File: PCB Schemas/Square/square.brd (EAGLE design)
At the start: 100 x 80 mm, 10 parts

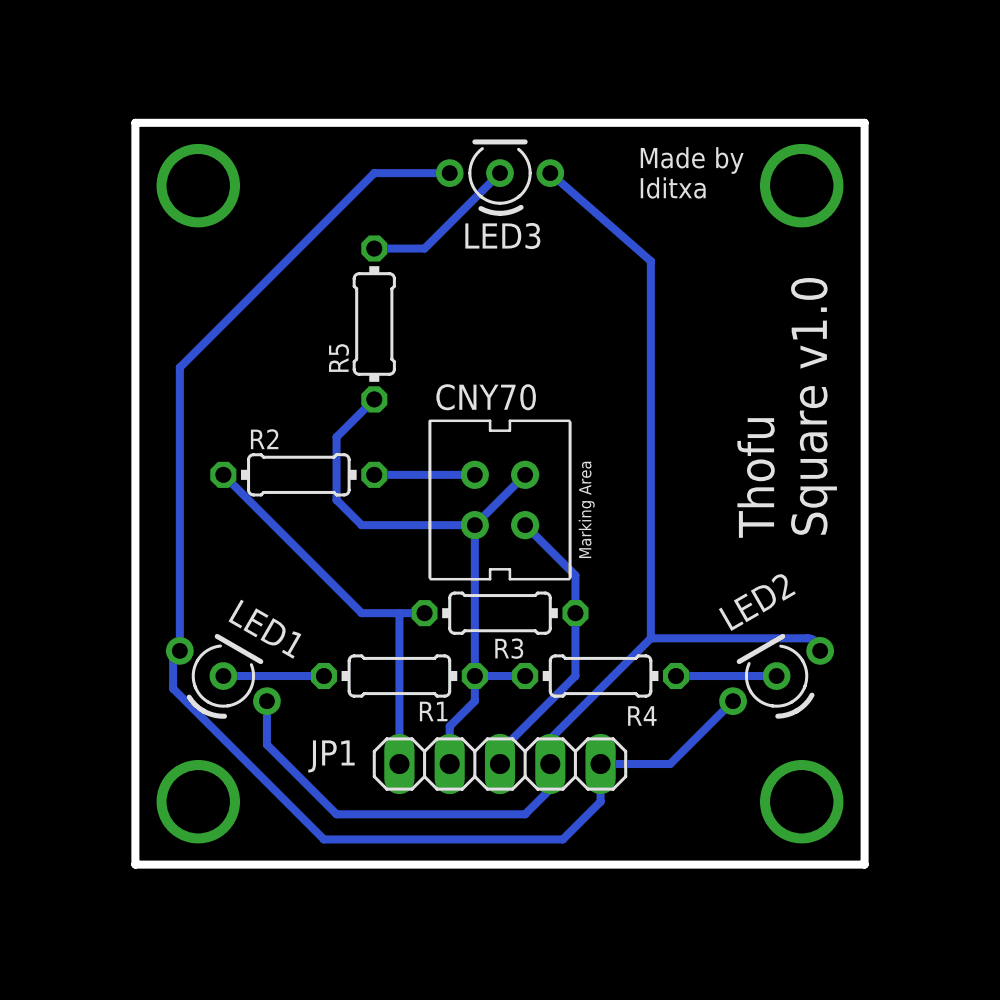
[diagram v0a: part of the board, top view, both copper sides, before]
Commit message: Updated and Finalized Square Board V1
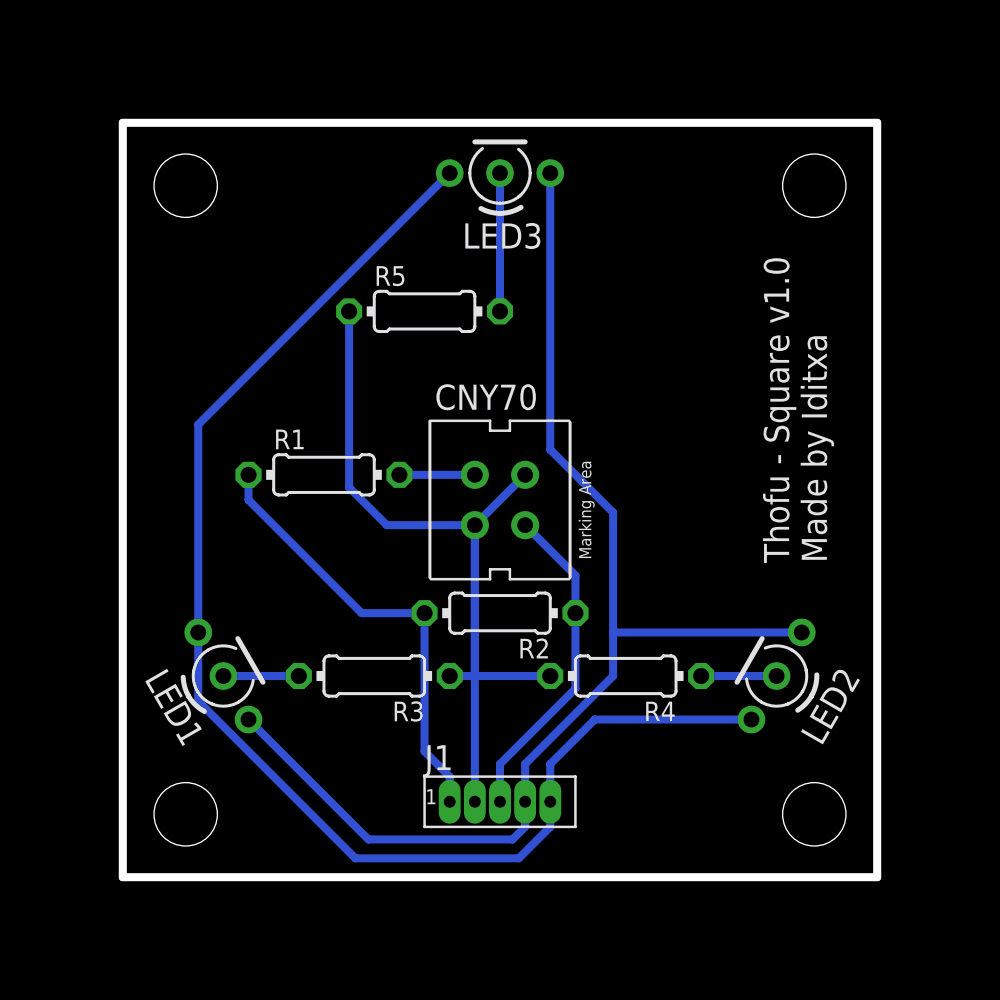
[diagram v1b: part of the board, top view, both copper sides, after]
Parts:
- removed JP1: (no value), pinhead:1X05
- added J1: (no value), Connectors:CON_5P_1.27
- R2: value 220 -> 10k
- R3: value 10k -> 220
- moved R2 12.3 mm to (61.0, 34.9), turned to 180 degrees
- moved R1 10.9 mm to (52.1, 41.9), turned to 0 degrees
- moved R3 7.10 mm to (54.6, 31.8)
- moved R5 2.62 mm to (57.1, 50.2), turned to 0 degrees
- moved R4 1.27 mm to (67.3, 31.8)
- turned LED1 to 300 degrees
- turned LED2 to 60 degrees
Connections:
- net COLOR: now also J1.3, R2.1; no longer JP1.3, R3.1
- net G: now also J1.5; no longer JP1.5
- net GND: now also J1.2, R3.1; no longer JP1.2, R1.1
- net N$1: now also R3.2; no longer R1.2
- net N$2: now also R1.2; no longer R2.2
- net R: now also J1.4; no longer JP1.4
- net VCC: now also J1.1, R1.1, R2.2; no longer JP1.1, R2.1, R3.2
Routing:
- net GND: track 32.1 -> 46.3 mm
- net VCC: track 20.7 -> 22.6 mm
- net COLOR: track 14.7 -> 16.6 mm
- net G: track 69.5 -> 67.9 mm
- net N$9: track 5.08 -> 3.81 mm
- net N$2: track 5.08 -> 3.81 mm
- net N$1: track 5.08 -> 3.81 mm
- net N$10: track 7.93 -> 6.98 mm
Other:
- outline, holes or cut-outs redrawn
- board text added: "Thofu - Square v1.0"
- board text removed: "Thofu Square v1.0"
